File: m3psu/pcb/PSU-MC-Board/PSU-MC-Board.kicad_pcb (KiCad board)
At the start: 2 copper layers, 40 x 40 mm, 56 parts, among them IC1 STM32F405RxTx, IC2 TPS62152, IC3 MCP2562, IC4 LTC4353, IC5 LTC4151, J1 WEST TOP, J2 WEST BOT, J3 NORTH TOP, J4 EAST TOP, J5 EAST BOT, J6 NORTH BOT, Q1 NFET, Q2 PFET, Q3 NFET, Q4 NFET2, Q5 NFET2, Q6 PFET, Q7 NFET, Q8 PFET, Q9 NFET, Y1 26M

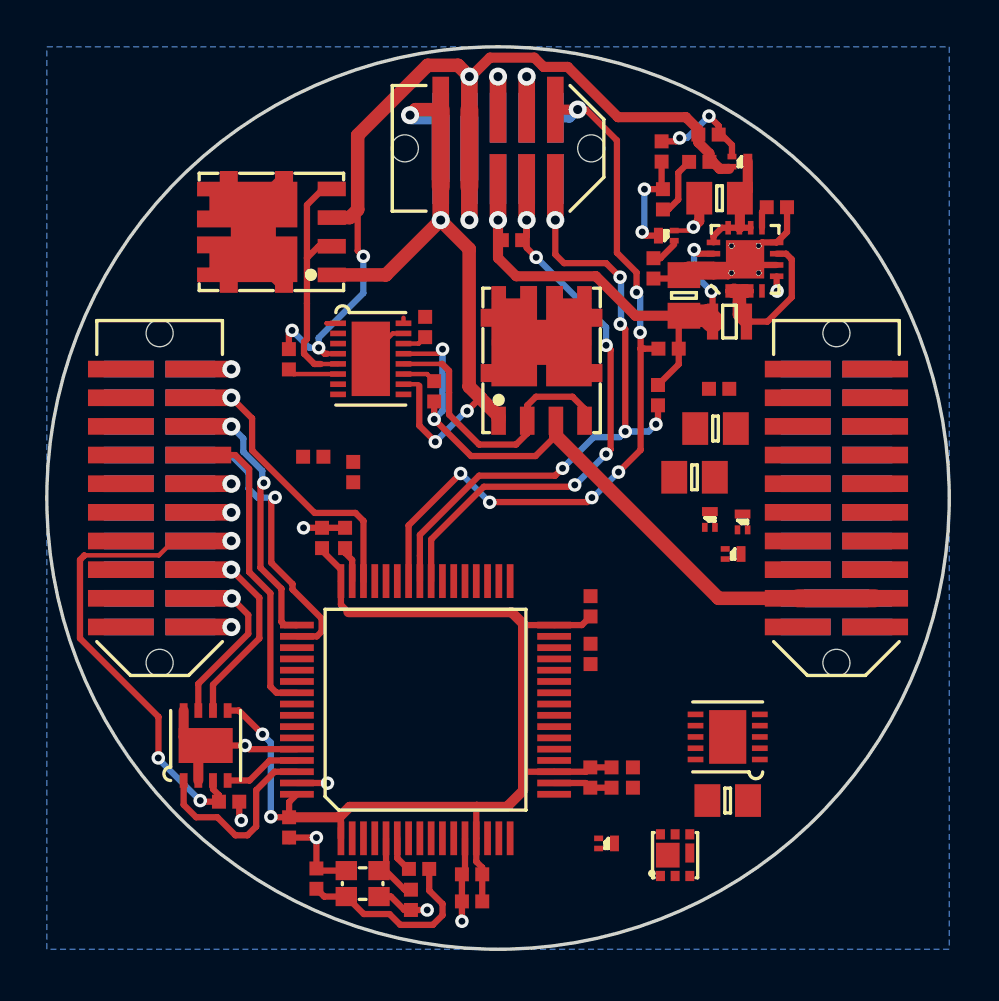
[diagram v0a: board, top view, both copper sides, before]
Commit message: Finished routing PSU uC board. Just needs checking.
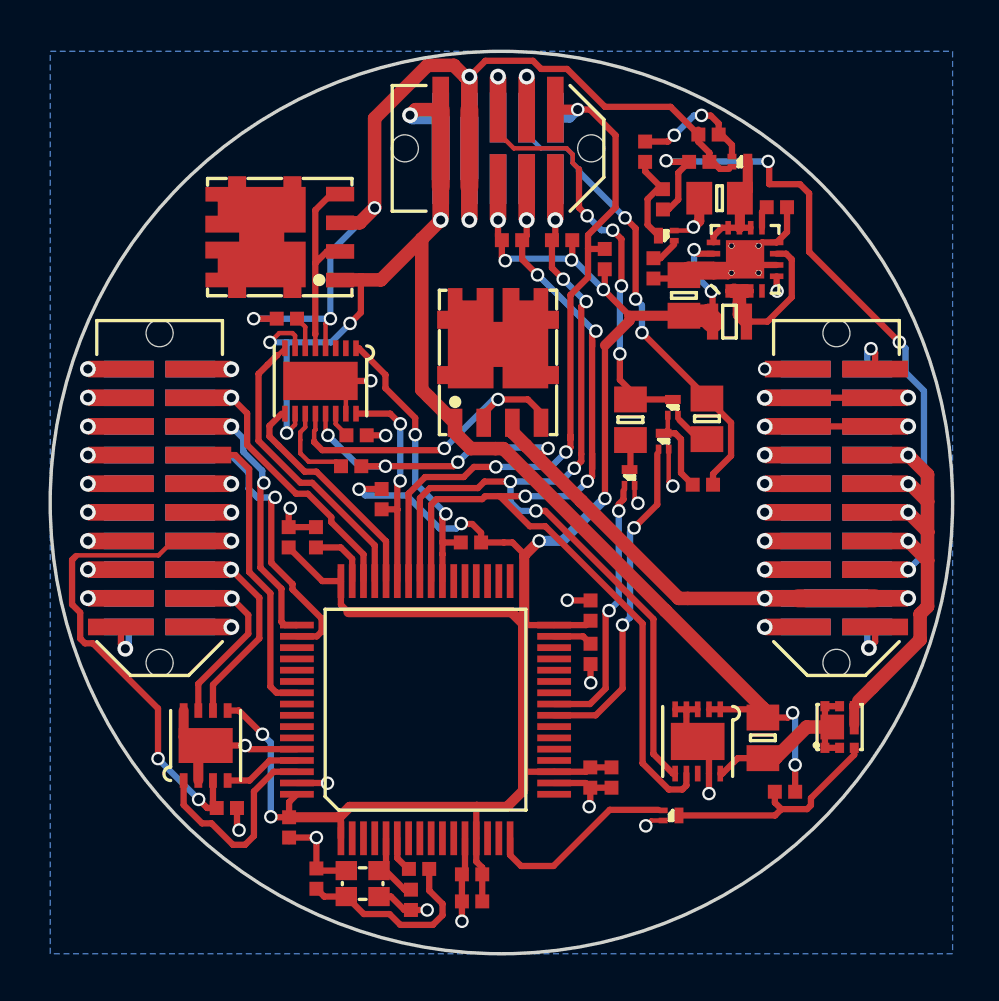
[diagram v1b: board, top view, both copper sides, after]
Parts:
- moved Q8 9.24 mm to (115.1, 110.2)
- moved R8 8.08 mm to (102.8, 88.6), turned to 180 degrees
- moved R11 7.96 mm to (98.8, 102.0)
- moved R16 6.77 mm to (112.7, 113.0), turned to 180 degrees
- moved Q3 5.87 mm to (107.3, 97.5), turned to 0 degrees
- moved C15 5.68 mm to (93.7, 97.2), turned to 0 degrees
- moved Q7 5.38 mm to (105.8, 99.1)
- moved Q6 5.23 mm to (107.8, 96.0)
- moved C17 4.96 mm to (93.5, 98.6), turned to 0 degrees
- moved R10 4.88 mm to (104.7, 89.4), turned to 90 degrees
- moved R12 4.31 mm to (109.1, 99.4), turned to 180 degrees
- moved R14 3.82 mm to (105.9, 96.5), turned to 270 degrees
- moved R15 3.19 mm to (111.7, 110.6), turned to 270 degrees
- moved Q9 3.12 mm to (107.7, 114.1)
- moved IC4 2.44 mm to (92.1, 94.8), turned to 270 degrees
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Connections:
- IC1 pad 16: Net-(IC1-Pad16) -> /EN_PYRO
- IC1 pad 24: Net-(IC1-Pad24) -> /BLEED_BATT2
- IC1 pad 25: Net-(IC1-Pad25) -> /BLEED_BATT1
- IC1 pad 39: Net-(IC1-Pad39) -> /~EN_INT_PWR
- IC1 pad 43: Net-(IC1-Pad43) -> /~EN_EXT_PWR
- IC1 pad 44: Net-(IC1-Pad44) -> /~EXT_PWR_ON
- IC1 pad 45: Net-(IC1-Pad45) -> /~INT_PWR_ON
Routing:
- net VCC: track 34.6 -> 67.2 mm, vias 4 -> 7
- net /PYRO1: track 0.00 -> 32.2 mm, vias 0 -> 4
- net /PWR: track 2.73 -> 33.6 mm, vias 0 -> 4
- net GND: track 50.3 -> 80.1 mm, vias 11 -> 26
- net 3v3: track 75.1 -> 100.5 mm, vias 5 -> 12
- net /BATT2: track 3.28 -> 24.3 mm, vias 1 -> 4
- net /BATT1: track 3.28 -> 22.2 mm, vias 1 -> 5
- net /SDA: track 27.4 -> 46.1 mm
- net /BLEED_BATT2: track 0.00 -> 14.8 mm, vias 0 -> 2
- net /~INT_PWR_ON: track 0.00 -> 13.3 mm
- net /~EN_INT_PWR: track 0.51 -> 13.0 mm, vias 0 -> 2
- net /BLEED_BATT1: track 0.00 -> 12.1 mm, vias 0 -> 2
- net /SCL: track 31.9 -> 43.0 mm
- net /~EXT_PWR_ON: track 0.00 -> 10.4 mm
- net Net-(Q8-PadG): track 0.00 -> 10.3 mm
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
